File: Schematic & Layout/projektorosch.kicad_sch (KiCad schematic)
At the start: 28 parts, among them J1 Barrel_Jack_Switch, J2 Conn_01x03, J3 RJ12, U1 ATtiny214-SS, U2 MAX232

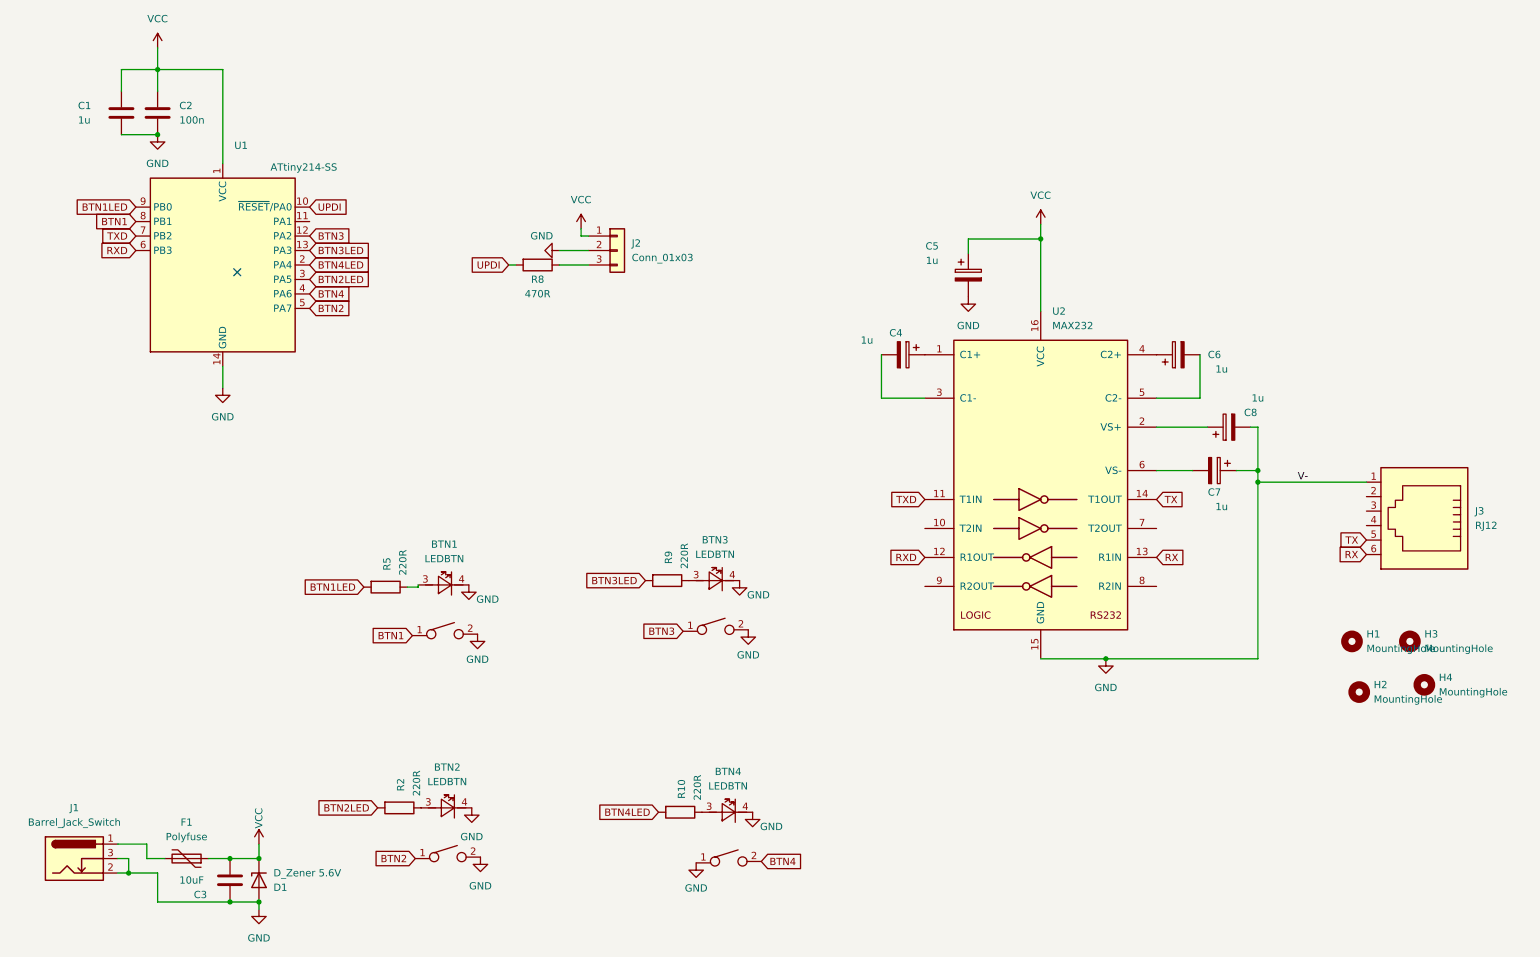
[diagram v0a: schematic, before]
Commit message: normal buttons
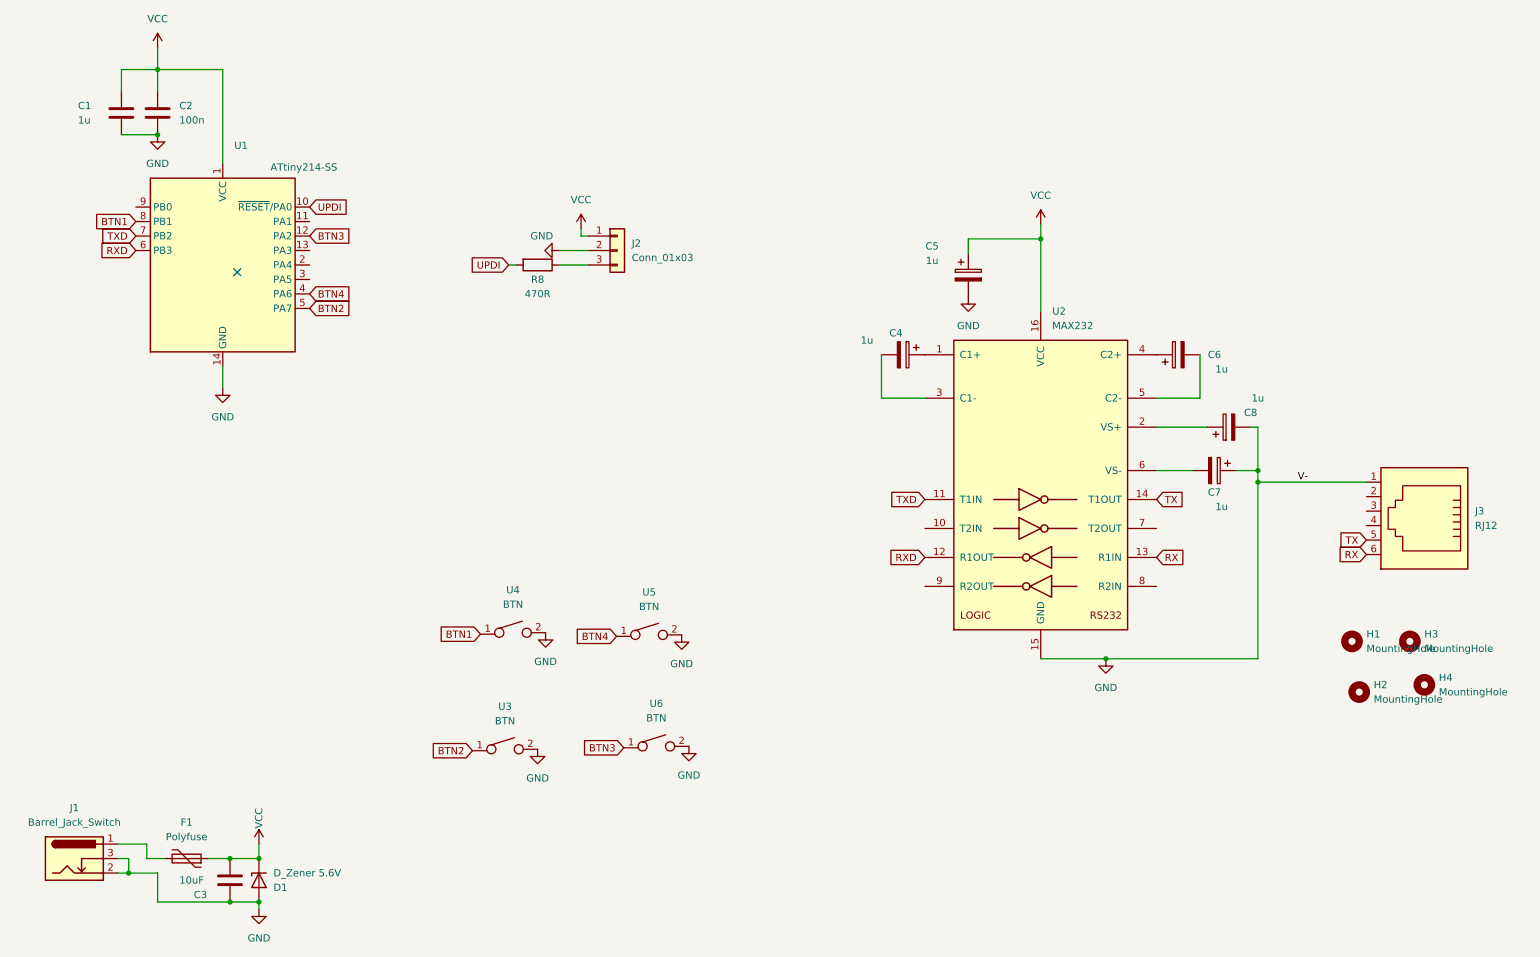
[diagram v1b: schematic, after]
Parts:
- removed BTN1, BTN2, BTN3, BTN4: LEDBTN, ledbtn_footprint:LBTN, symbol projektorosch:LEDBTN
- removed R10, R2, R5, R9: 220R, Resistor_SMD:R_0805_2012Metric_Pad1.20x1.40mm_HandSolder, symbol Device:R
- added U3, U4, U5, U6: BTN, Button_Switch_THT:SW_PUSH_6mm_H5mm, symbol projektorosch:BTN
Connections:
- net BTN1: now also U4.1
- net BTN2: now also U3.1
- net BTN3: now also U6.1
- net BTN4: now also U5.1
- net GND: now also U3.2, U4.2, U5.2, U6.2
- net BTN1LED: no longer names the net of U1.9 (PB0)
- net BTN2LED: no longer names the net of U1.3 (PA5)
- net BTN3LED: no longer names the net of U1.13 (PA3)
- net BTN4LED: no longer names the net of U1.2 (PA4)
